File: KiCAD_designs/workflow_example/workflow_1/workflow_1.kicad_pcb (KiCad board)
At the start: 2 copper layers, 21 x 18 mm, 5 parts, among them J1 B2B-PH-SM4-TBLFSN, SW1 CUS-12TB, U1 ATTINY45-20SU

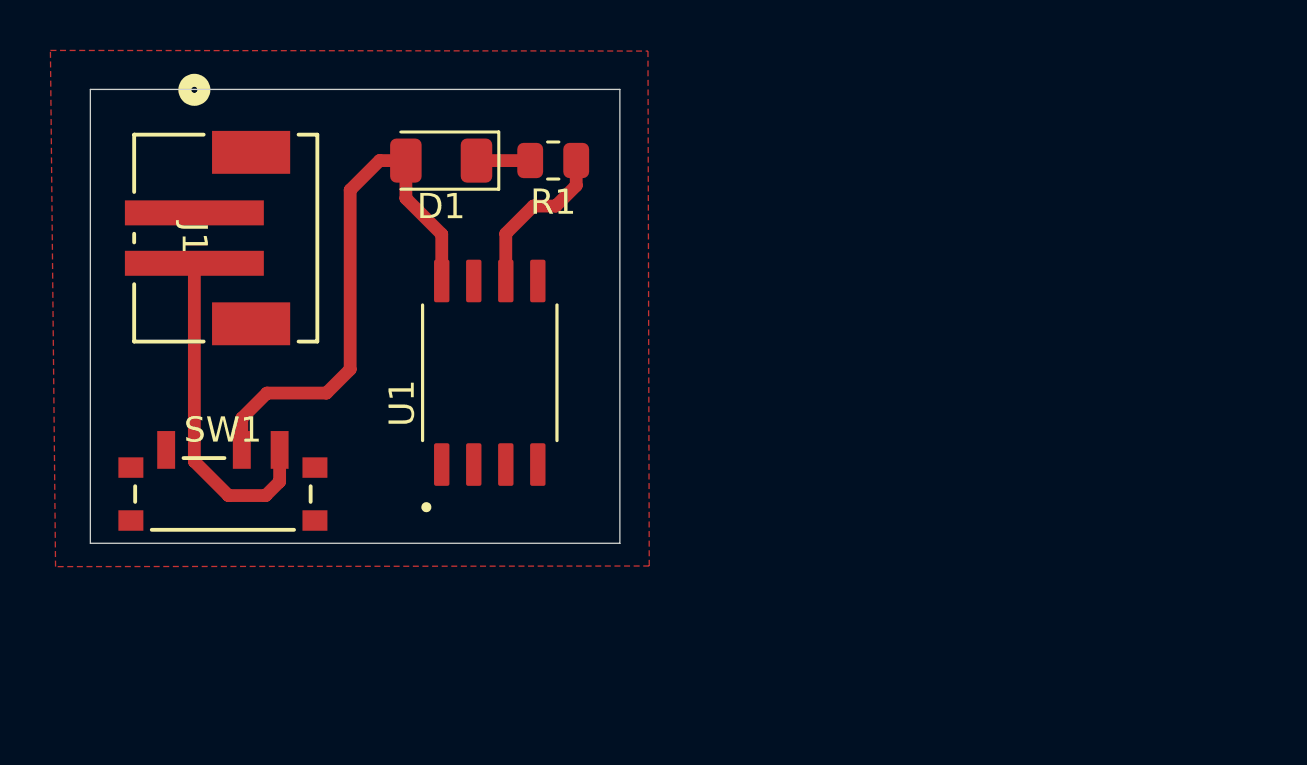
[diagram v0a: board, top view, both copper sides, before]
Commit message: misalign
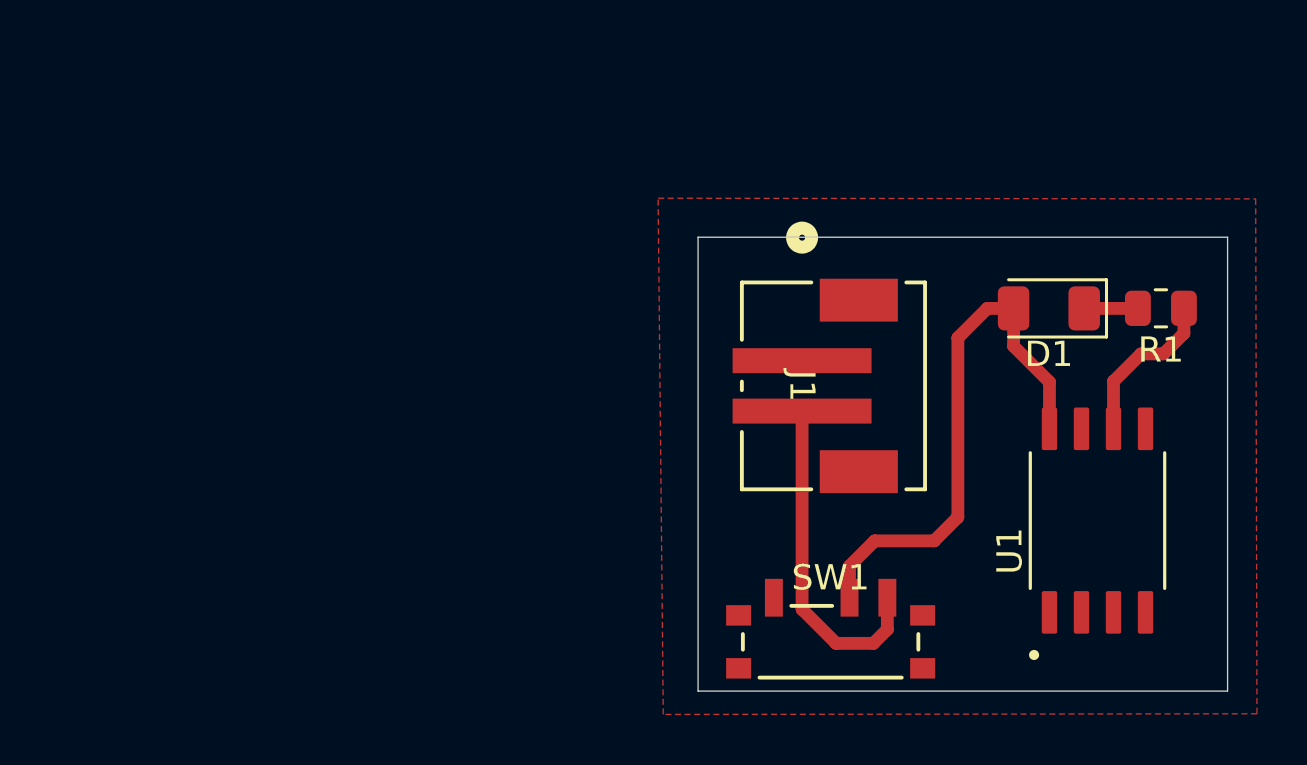
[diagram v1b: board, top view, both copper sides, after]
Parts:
- moved D1 24.8 mm to (120.0, 59.7)
- moved J1 24.8 mm to (111.5, 62.8)
- moved R1 24.8 mm to (124.5, 59.7)
- moved SW1 24.8 mm to (111.4, 72.9)
- moved U1 24.8 mm to (121.9, 68.1)
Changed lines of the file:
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@@
   (net 10 "/vin")
   (footprint "LED_SMD:LED_1206_3216Metric" (layer "F.Cu")
-    (at 95.9134 53.8226 180)
+    (at 120.015 59.6848 180)
     (descr "LED SMD 1206 (3216 Metric), square (rectangular) end terminal, IPC_7351 nominal, (Body size source: http://www.tortai-tech.com/upload/download/2011102023233369053.pdf), generated with kicad-footprint-generator")
     (tags "LED")
@@
   )
   (footprint "Library:SOIC127P794X202-8N" (layer "F.Cu")
-    (at 97.8408 62.2378 90)
+    (at 121.9424 68.1 90)
     (property "Availability" "")
     (property "Check_prices" "")
@@
   )
   (footprint "Resistor_SMD:R_0805_2012Metric" (layer "F.Cu")
-    (at 100.3565 53.8196 180)
+    (at 124.4581 59.6818 180)
     (descr "Resistor SMD 0805 (2012 Metric), square (rectangular) end terminal, IPC_7351 nominal, (Body size source: IPC-SM-782 page 72, https://www.pcb-3d.com/wordpress/wp-content/uploads/ipc-sm-782a_amendment_1_and_2.pdf), generated with kicad-footprint-generator")
     (tags "resistor")
@@
   )
   (footprint "esp_lib:B2B-PH-SM4-TBLFSN_JST" (layer "F.Cu")
-    (at 87.369751 56.896 -90)
+    (at 111.471351 62.7582 -90)
     (tags "B2B-PH-SM4-TBLFSN ")
     (property "Sheetfile" "workflow_1.kicad_sch")
@@
   )
   (footprint "Library:CUS-12TB_NDC" (layer "F.Cu")
-    (at 87.25662 67.042801)
+    (at 111.35822 72.905001)
     (tags "CUS-12TB ")
     (property "Sheetfile" "workflow_1.kicad_sch")
@@
     (pad "7" smd rect (at 3.64998 1.054599) (size 0.9906 0.8128) (layers "F.Cu" "F.Paste" "F.Mask"))
   )
-  (gr_rect (start 82 51) (end 103 69)
+  (gr_rect (start 106.1016 56.8622) (end 127.1016 74.8622)
     (stroke (width 0.05) (type default)) (fill none) (layer "Edge.Cuts"))
-  (segment (start 99.441 53.8226) (end 99.444 53.8196) (width 0.508) (layer "F.Cu") (net 1))
-  (segment (start 97.3134 53.8226) (end 99.441 53.8226) (width 0.508) (layer "F.Cu") (net 1))
-  (segment (start 88.00662 64.040101) (end 89.003921 63.0428) (width 0.508) (layer "F.Cu") (net 2))
-  (segment (start 92.3036 62.103) (end 92.3036 54.991) (width 0.508) (layer "F.Cu") (net 2))
-  (segment (start 95.9358 56.7436) (end 95.9358 58.5978) (width 0.508) (layer "F.Cu") (net 2))
-  (segment (start 91.3638 63.0428) (end 92.3036 62.103) (width 0.508) (layer "F.Cu") (net 2))
-  (segment (start 88.00662 65.297401) (end 88.00662 64.040101) (width 0.508) (layer "F.Cu") (net 2))
-  (segment (start 89.003921 63.0428) (end 91.3638 63.0428) (width 0.508) (layer "F.Cu") (net 2))
-  (segment (start 93.472 53.8226) (end 94.5134 53.8226) (width 0.508) (layer "F.Cu") (net 2))
-  (segment (start 94.5134 55.3212) (end 95.9358 56.7436) (width 0.508) (layer "F.Cu") (net 2))
-  (segment (start 92.3036 54.991) (end 93.472 53.8226) (width 0.508) (layer "F.Cu") (net 2))
-  (segment (start 94.5134 53.8226) (end 94.5134 55.3212) (width 0.508) (layer "F.Cu") (net 2))
-  (segment (start 101.269 53.8196) (end 101.269 54.814) (width 0.508) (layer "F.Cu") (net 4))
-  (segment (start 99.568 55.626) (end 98.4758 56.7182) (width 0.508) (layer "F.Cu") (net 4))
-  (segment (start 101.269 54.814) (end 100.457 55.626) (width 0.508) (layer "F.Cu") (net 4))
-  (segment (start 98.4758 56.7182) (end 98.4758 58.5978) (width 0.508) (layer "F.Cu") (net 4))
-  (segment (start 100.457 55.626) (end 99.568 55.626) (width 0.508) (layer "F.Cu") (net 4))
-  (segment (start 87.4776 67.1068) (end 88.954521 67.1068) (width 0.508) (layer "F.Cu") (net 10))
-  (segment (start 86.12495 57.896001) (end 86.12495 65.75415) (width 0.508) (layer "F.Cu") (net 10))
-  (segment (start 88.954521 67.1068) (end 89.50662 66.554701) (width 0.508) (layer "F.Cu") (net 10))
-  (segment (start 86.12495 65.75415) (end 87.4776 67.1068) (width 0.508) (layer "F.Cu") (net 10))
-  (segment (start 89.50662 66.554701) (end 89.50662 65.297401) (width 0.508) (layer "F.Cu") (net 10))
+  (segment (start 123.5426 59.6848) (end 123.5456 59.6818) (width 0.508) (layer "F.Cu") (net 1))
+  (segment (start 121.415 59.6848) (end 123.5426 59.6848) (width 0.508) (layer "F.Cu") (net 1))
+  (segment (start 112.10822 69.902301) (end 113.105521 68.905) (width 0.508) (layer "F.Cu") (net 2))
+  (segment (start 116.4052 67.9652) (end 116.4052 60.8532) (width 0.508) (layer "F.Cu") (net 2))
+  (segment (start 120.0374 62.6058) (end 120.0374 64.46) (width 0.508) (layer "F.Cu") (net 2))
+  (segment (start 115.4654 68.905) (end 116.4052 67.9652) (width 0.508) (layer "F.Cu") (net 2))
+  (segment (start 112.10822 71.159601) (end 112.10822 69.902301) (width 0.508) (layer "F.Cu") (net 2))
+  (segment (start 113.105521 68.905) (end 115.4654 68.905) (width 0.508) (layer "F.Cu") (net 2))
+  (segment (start 117.5736 59.6848) (end 118.615 59.6848) (width 0.508) (layer "F.Cu") (net 2))
+  (segment (start 118.615 61.1834) (end 120.0374 62.6058) (width 0.508) (layer "F.Cu") (net 2))
+  (segment (start 116.4052 60.8532) (end 117.5736 59.6848) (width 0.508) (layer "F.Cu") (net 2))
+  (segment (start 118.615 59.6848) (end 118.615 61.1834) (width 0.508) (layer "F.Cu") (net 2))
+  (segment (start 125.3706 59.6818) (end 125.3706 60.6762) (width 0.508) (layer "F.Cu") (net 4))
+  (segment (start 123.6696 61.4882) (end 122.5774 62.5804) (width 0.508) (layer "F.Cu") (net 4))
+  (segment (start 125.3706 60.6762) (end 124.5586 61.4882) (width 0.508) (layer "F.Cu") (net 4))
+  (segment (start 122.5774 62.5804) (end 122.5774 64.46) (width 0.508) (layer "F.Cu") (net 4))
+  (segment (start 124.5586 61.4882) (end 123.6696 61.4882) (width 0.508) (layer "F.Cu") (net 4))
+  (segment (start 111.5792 72.969) (end 113.056121 72.969) (width 0.508) (layer "F.Cu") (net 10))
+  (segment (start 110.22655 63.758201) (end 110.22655 71.61635) (width 0.508) (layer "F.Cu") (net 10))
+  (segment (start 113.056121 72.969) (end 113.60822 72.416901) (width 0.508) (layer "F.Cu") (net 10))
+  (segment (start 110.22655 71.61635) (end 111.5792 72.969) (width 0.508) (layer "F.Cu") (net 10))
+  (segment (start 113.60822 72.416901) (end 113.60822 71.159601) (width 0.508) (layer "F.Cu") (net 10))
   (zone (net 3) (net_name "/GND") (layer "F.Cu") (hatch edge 0.5)
     (connect_pads (clearance 0.5))
@@
     (polygon
       (pts
-        (xy 80.4164 49.4538)
-        (xy 104.1146 49.4792)
-        (xy 104.1654 69.9008)
-        (xy 80.6196 69.9262)
+        (xy 104.518 55.316)
+        (xy 128.2162 55.3414)
+        (xy 128.267 75.763)
+        (xy 104.7212 75.7884)
       )
     )
